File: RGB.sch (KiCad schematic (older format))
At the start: 25 parts

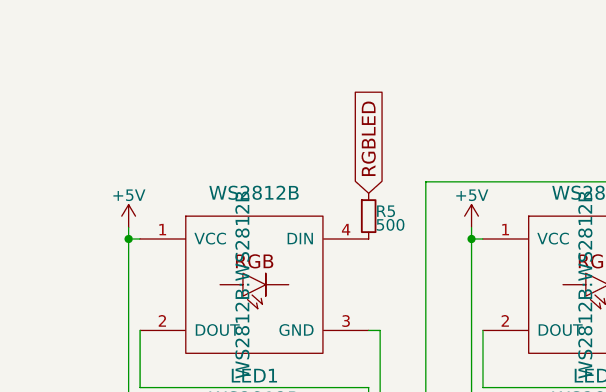
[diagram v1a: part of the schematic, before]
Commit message: Fix RGB voltage
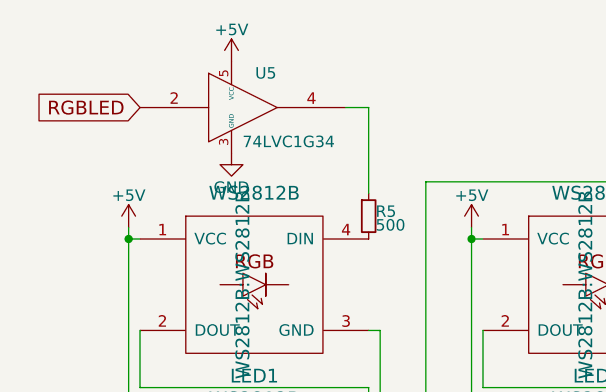
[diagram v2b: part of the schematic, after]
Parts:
- added U5: 74LVC1G34, TO_SOT_Packages_SMD:SOT-353_SC-70-5, symbol 74LVC1G34
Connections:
- net +5V: now also U5.5 (VCC)
- net GND: now also U5.3 (GND)
- net RGBLED: now also U5.2; no longer R5.1
- new net: R5.1, U5.4
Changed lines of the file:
@@
 LIBS:Tag-Connect
 LIBS:ai03-locallib
+LIBS:logic
 LIBS:VoyagerII-cache
 EELAYER 25 0
@@
 	1    0    0    -1
 $EndComp
-Text GLabel 2775 1325 1    60   Input ~ 0
+Text GLabel 1775 950  0    60   Input ~ 0
 RGBLED
 $Comp
-L GND #PWR021
+L GND #PWR27
 U 1 1 5A6B55C8
 P 2825 6475
-F 0 "#PWR021" H 2825 6225 50  0001 C CNN
+F 0 "#PWR27" H 2825 6225 50  0001 C CNN
 F 1 "GND" H 2825 6325 50  0000 C CNN
 F 2 "" H 2825 6475 50  0001 C CNN
@@
 $EndComp
 $Comp
-L +5V #PWR022
+L +5V #PWR23
 U 1 1 5A6B5B93
 P 1725 1475
-F 0 "#PWR022" H 1725 1325 50  0001 C CNN
+F 0 "#PWR23" H 1725 1325 50  0001 C CNN
 F 1 "+5V" H 1725 1615 50  0000 C CNN
 F 2 "" H 1725 1475 50  0001 C CNN
@@
 $EndComp
 $Comp
-L GND #PWR023
+L GND #PWR28
 U 1 1 5A6B6273
 P 4325 6475
-F 0 "#PWR023" H 4325 6225 50  0001 C CNN
+F 0 "#PWR28" H 4325 6225 50  0001 C CNN
 F 1 "GND" H 4325 6325 50  0000 C CNN
 F 2 "" H 4325 6475 50  0001 C CNN
@@
 NoConn ~ 3275 6425
 $Comp
-L +5V #PWR024
+L +5V #PWR24
 U 1 1 5A6B6BA2
 P 3225 1475
-F 0 "#PWR024" H 3225 1325 50  0001 C CNN
+F 0 "#PWR24" H 3225 1325 50  0001 C CNN
 F 1 "+5V" H 3225 1615 50  0000 C CNN
 F 2 "" H 3225 1475 50  0001 C CNN
@@
 Connection ~ 5675 2450
 $Comp
-L GND #PWR025
+L GND #PWR26
 U 1 1 5A6B9075
 P 5550 2775
-F 0 "#PWR025" H 5550 2525 50  0001 C CNN
+F 0 "#PWR26" H 5550 2525 50  0001 C CNN
 F 1 "GND" H 5550 2625 50  0000 C CNN
 F 2 "" H 5550 2775 50  0001 C CNN
@@
 $EndComp
 $Comp
-L +5V #PWR026
+L +5V #PWR25
 U 1 1 5A6B90B9
 P 5475 2250
-F 0 "#PWR026" H 5475 2100 50  0001 C CNN
+F 0 "#PWR25" H 5475 2100 50  0001 C CNN
 F 1 "+5V" H 5475 2390 50  0000 C CNN
 F 2 "" H 5475 2250 50  0001 C CNN
@@
 	1    0    0    -1
 $EndComp
+$Comp
+L 74LVC1G34 U5
+U 1 1 5A6EE85D
+P 2225 950
+F 0 "U5" H 2325 1100 50  0000 C CNN
+F 1 "74LVC1G34" H 2425 800 50  0000 C CNN
+F 2 "TO_SOT_Packages_SMD:SOT-353_SC-70-5" H 2225 950 50  0001 C CNN
+F 3 "" H 2225 950 50  0001 C CNN
+	1    2225 950
+	1    0    0    -1
+$EndComp
+Wire Wire Line
+	2675 950  2775 950
+Wire Wire Line
+	2775 950  2775 1325
+$Comp
+L +5V #PWR21
+U 1 1 5A6EEA29
+P 2175 750
+F 0 "#PWR21" H 2175 600 50  0001 C CNN
+F 1 "+5V" H 2175 890 50  0000 C CNN
+F 2 "" H 2175 750 50  0001 C CNN
+F 3 "" H 2175 750 50  0001 C CNN
+	1    2175 750
+	1    0    0    -1
+$EndComp
+$Comp
+L GND #PWR22
+U 1 1 5A6EEA71
+P 2175 1150
+F 0 "#PWR22" H 2175 900 50  0001 C CNN
+F 1 "GND" H 2175 1000 50  0000 C CNN
+F 2 "" H 2175 1150 50  0001 C CNN
+F 3 "" H 2175 1150 50  0001 C CNN
+	1    2175 1150
+	1    0    0    -1
+$EndComp
